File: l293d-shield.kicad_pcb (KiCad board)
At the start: 2 copper layers, 53.3 x 43.2 mm, 4 parts, among them J1 CONN_01X04, J2 CONN_01X02, U1 l293d

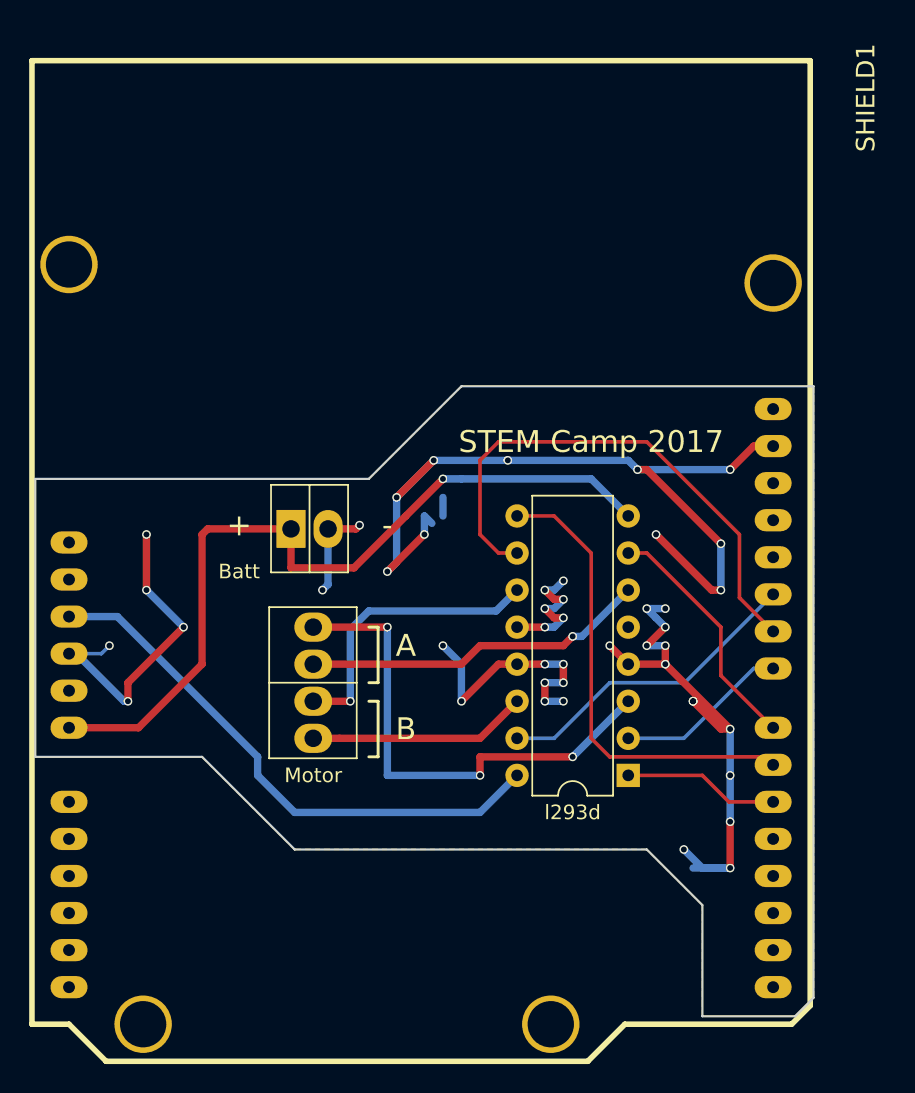
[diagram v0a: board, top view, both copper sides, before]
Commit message: Generaate output files
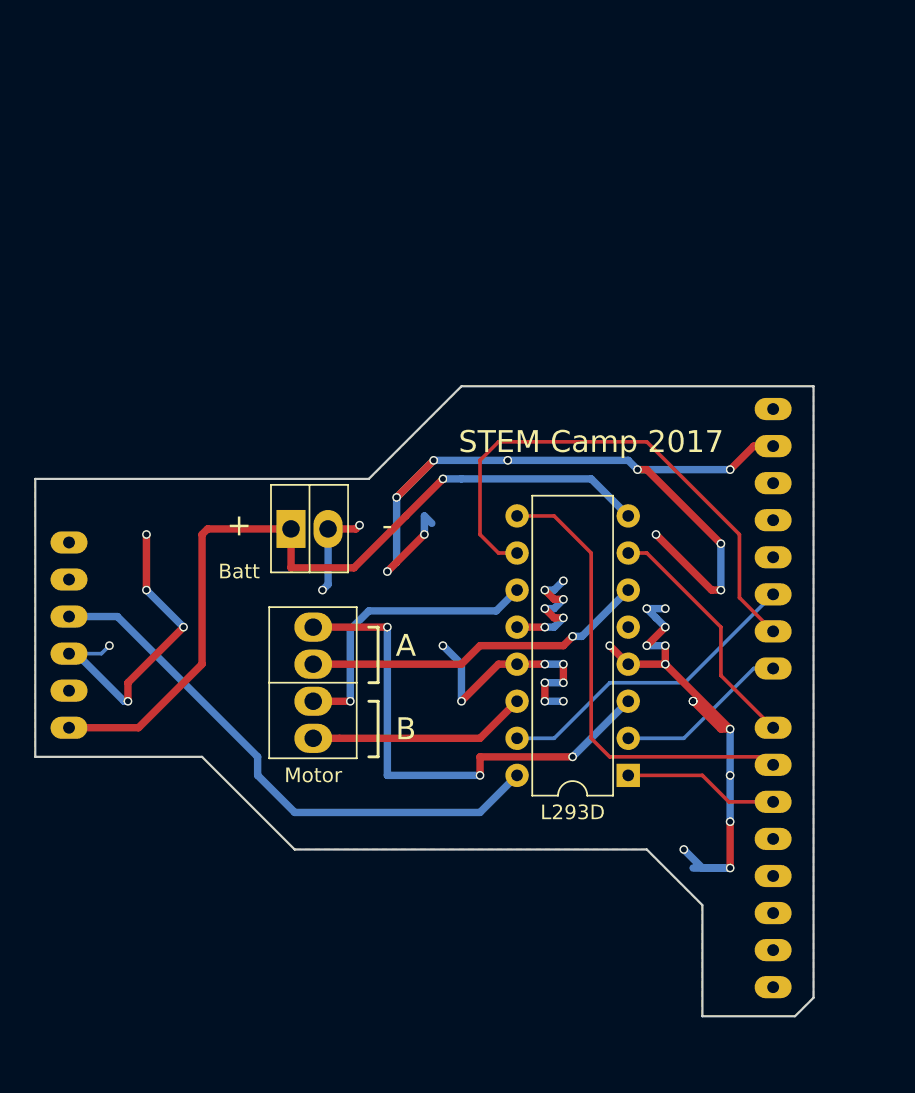
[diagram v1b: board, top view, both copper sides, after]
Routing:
- net (no net): track 1.27 -> 0.00 mm
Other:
- board text added: "L293D"
- board text removed: "l293d"
